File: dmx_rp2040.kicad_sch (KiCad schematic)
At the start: 8 parts, among them J1 XLR3_IN, J2 XLR3_OUT, SW1 SW_Push, U1 MAX485E

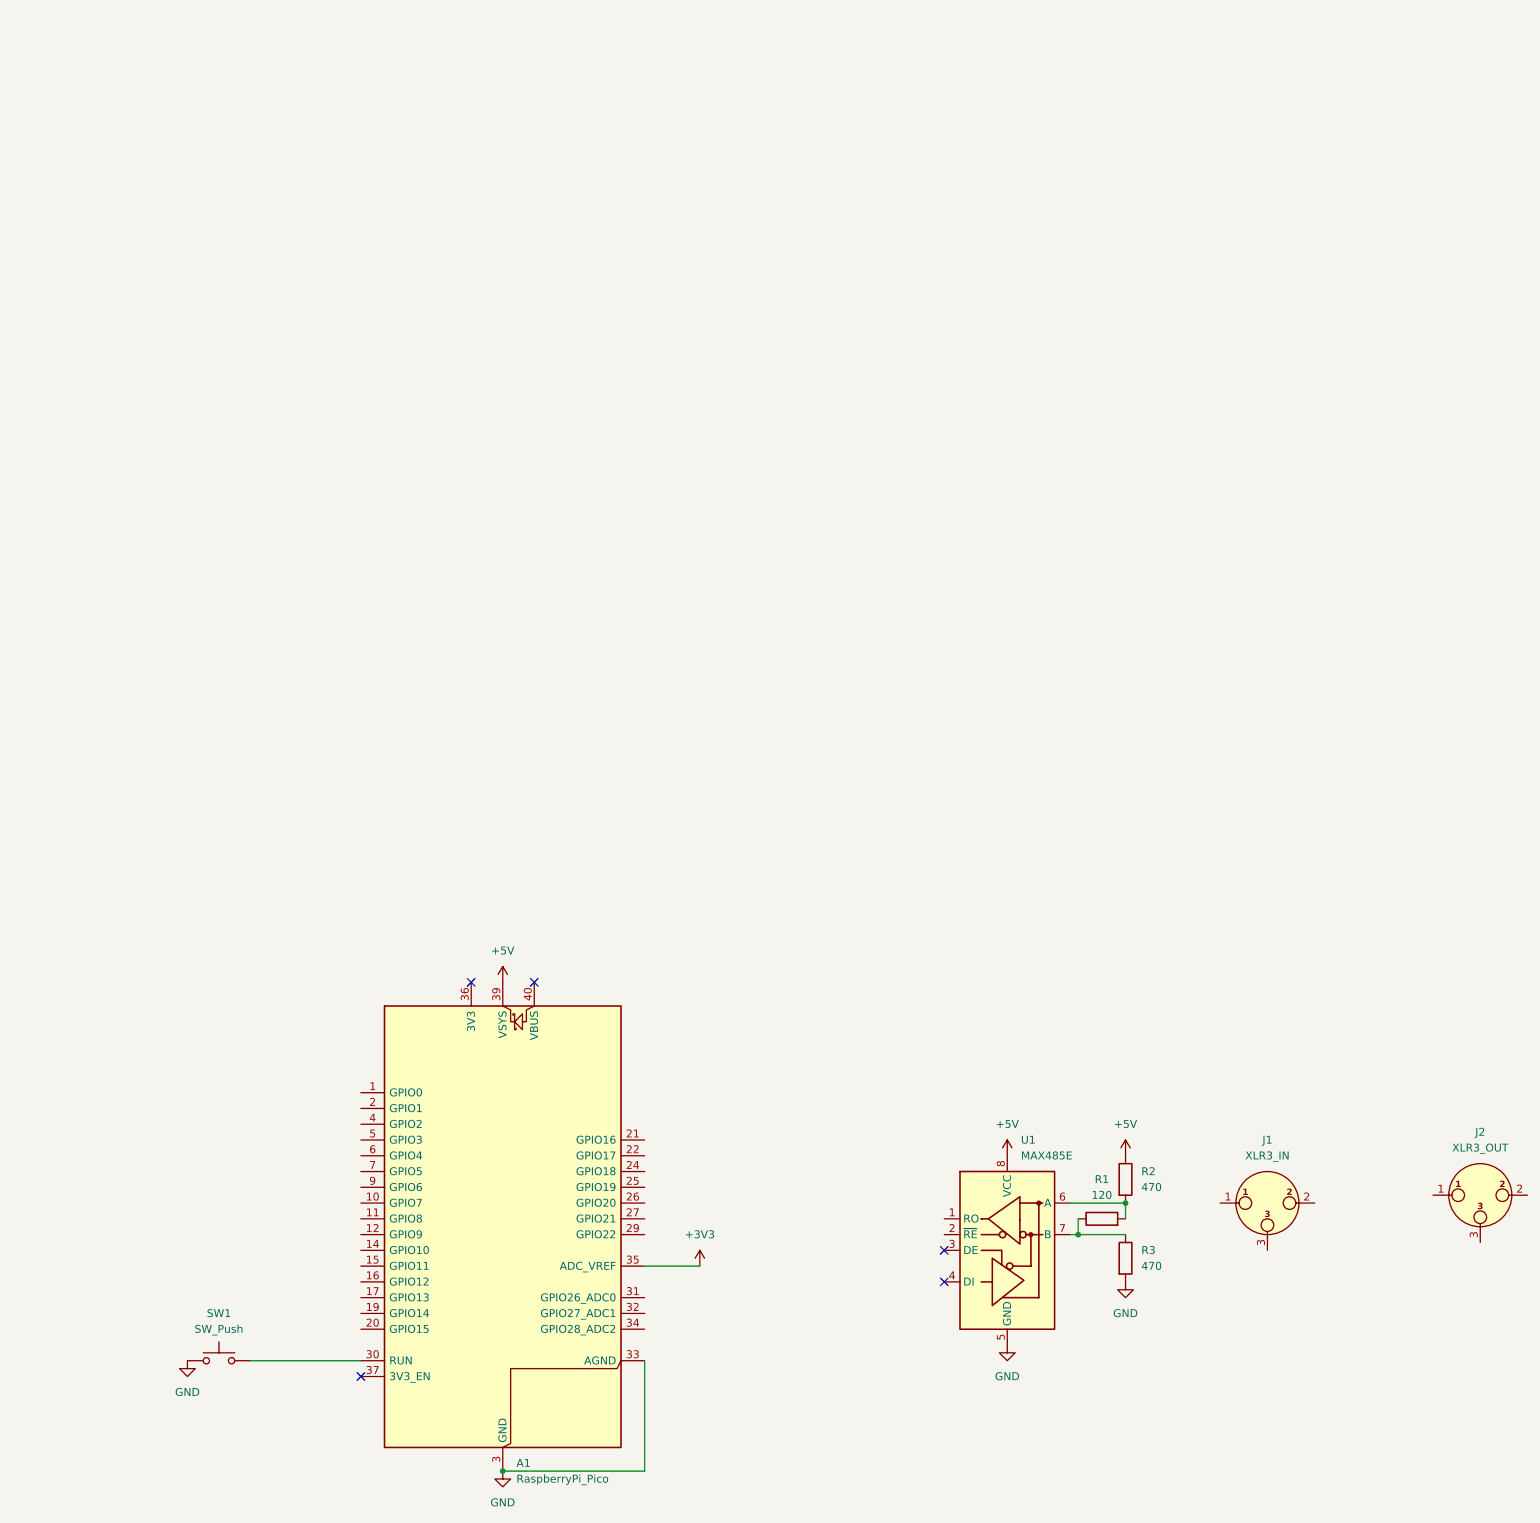
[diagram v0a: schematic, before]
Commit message: redid everything. works better now
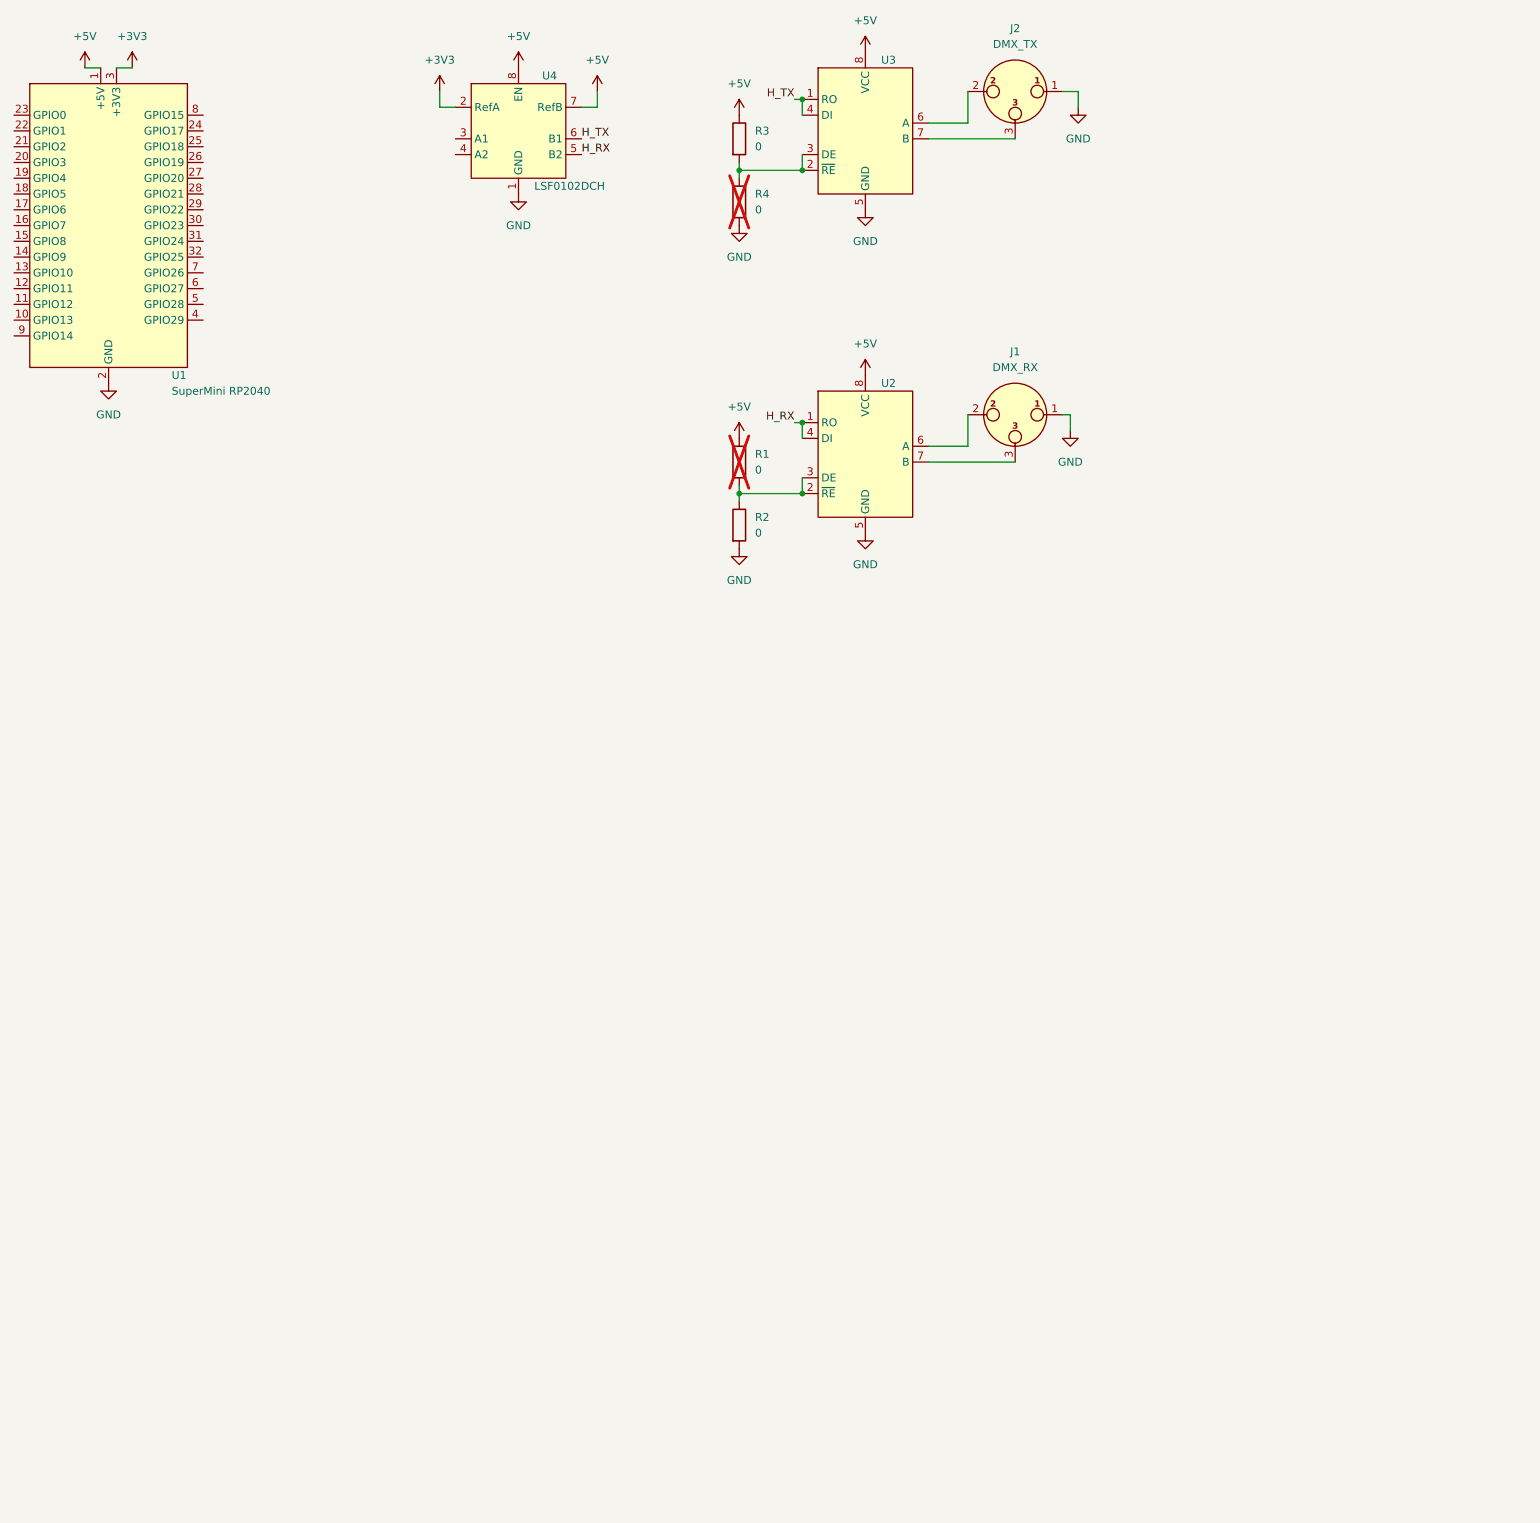
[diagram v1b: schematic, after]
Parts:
- removed A1: RaspberryPi_Pico, Module_RaspberryPi_Pico:RaspberryPi_Pico_Common_SMD, symbol MCU_Module_RaspberryPi_Pico:RaspberryPi_Pico
- removed SW1: SW_Push, symbol Switch:SW_Push
- removed U1: MAX485E, Package_SO:SOIC-8_3.9x4.9mm_P1.27mm, symbol Interface_UART:MAX485E
- added R4: 0, symbol Device:R
- added U1: SuperMini RP2040, symbol _symbols:SuperMini_RP2040
- added U2, U3: (no value), Package_SO:SOIC-8_5.3x6.2mm_P1.27mm, symbol _symbols:DS485MX
- added U4: LSF0102DCH, Package_SO:VSSOP-8_2.3x2mm_P0.5mm, symbol _symbols:LSF0102DCH
- J1: value XLR3_IN -> DMX_RX
- J2: value XLR3_OUT -> DMX_TX
- R1: value 120 -> 0; now not fitted
- R2, R3: value 470 -> 0
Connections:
- net +3V3: now also U1.3 (+3V3), U4.2 (RefA)
- net +5V: now also R1.1, R3.1, U1.1 (+5V), U2.8 (VCC), U3.8 (VCC), U4.7 (RefB), U4.8 (EN); no longer R2.1
- net GND: now also J1.1, J2.1, R2.2, R4.2, U1.2 (GND), U1.33 (GND), U2.5 (GND), U3.5 (GND), U4.1 (GND); no longer R3.2
- net at R1.2: now also R2.1, U2.2 (~{RE}), U2.3 (DE); no longer R2.2
- net at J1.2: now also U2.6 (A)
- net at J1.3: now also U2.7 (B)
- net at J2.2: now also U3.6 (A)
- net at J2.3: now also U3.7 (B)
- new net: R3.2, R4.1, U3.2 (~{RE}), U3.3 (DE)
- new net H_RX: U2.1 (RO), U2.4 (DI), U4.5 (B2)
- new net H_TX: U3.1 (RO), U3.4 (DI), U4.6 (B1)
- no-connect marks 5 -> 0
